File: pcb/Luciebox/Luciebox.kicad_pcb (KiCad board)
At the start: 2 copper layers, 100 x 100 mm, 96 parts, among them J1 Screw_Terminal_01x07, J2 Screw_Terminal_01x07, J3 Screw_Terminal_01x07, J4 Screw_Terminal_01x07, J5 Screw_Terminal_01x07, P1 CONN_01X01, P2 CONN_01X01, P3 CONN_01X01, P4 CONN_01X01, P5 Digital, P6 Power, P7 Digital, P8 Analog, Q1 BC558, Q2 N-Channel_Mosfet, T1 terminal_13x1, T10 terminal_8x1, T11 terminal_3x1, T2 terminal_8x1, T3 terminal_8x1, T4 terminal_8x1, T5 terminal_8x1, T6 terminal_8x1, T7 terminal_8x1, T8 terminal_8x1, T9 terminal_8x1, U1 CA56-12SRWA, U2 ULN2003A, U3 ATmega328-PU, U4 8X8PADS, Y1 16MHz

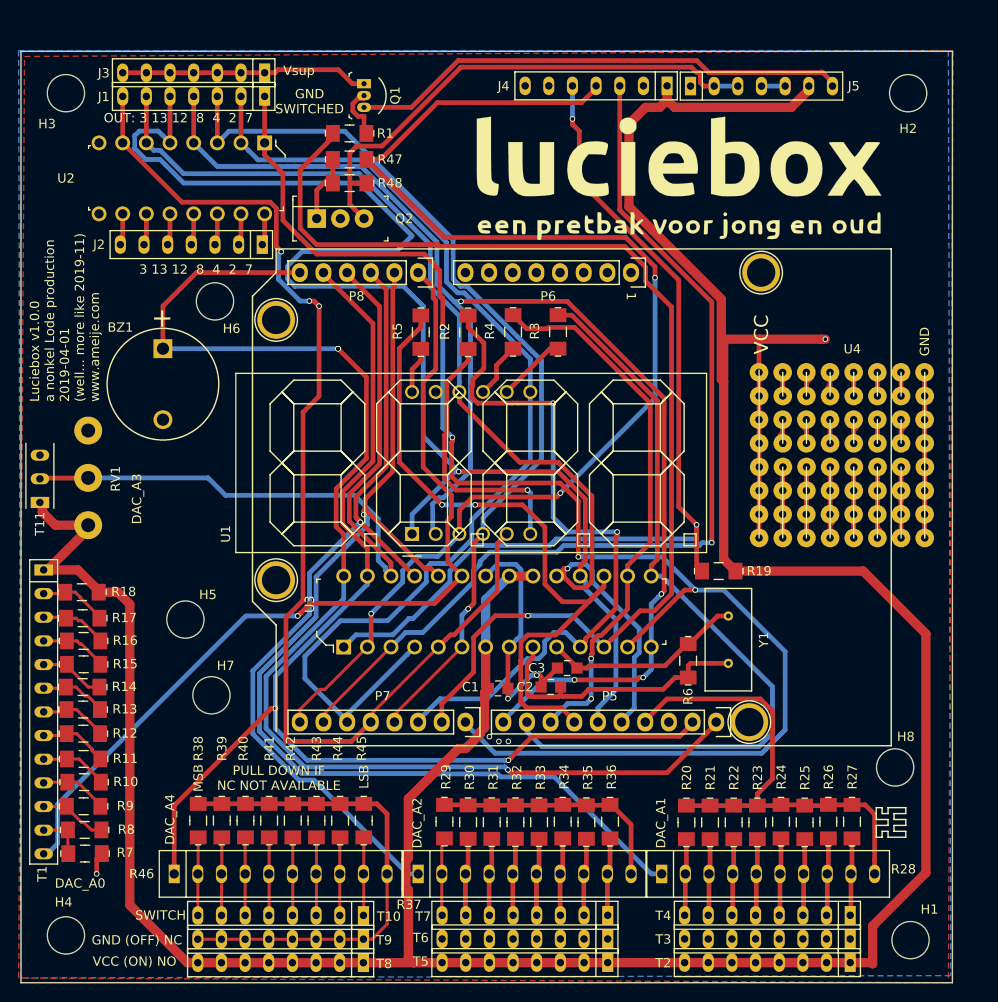
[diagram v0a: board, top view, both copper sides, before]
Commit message: reload autosave, the v1.0.0 save was not actually saved. oioioi. So, now at v1.0.0 pcb!
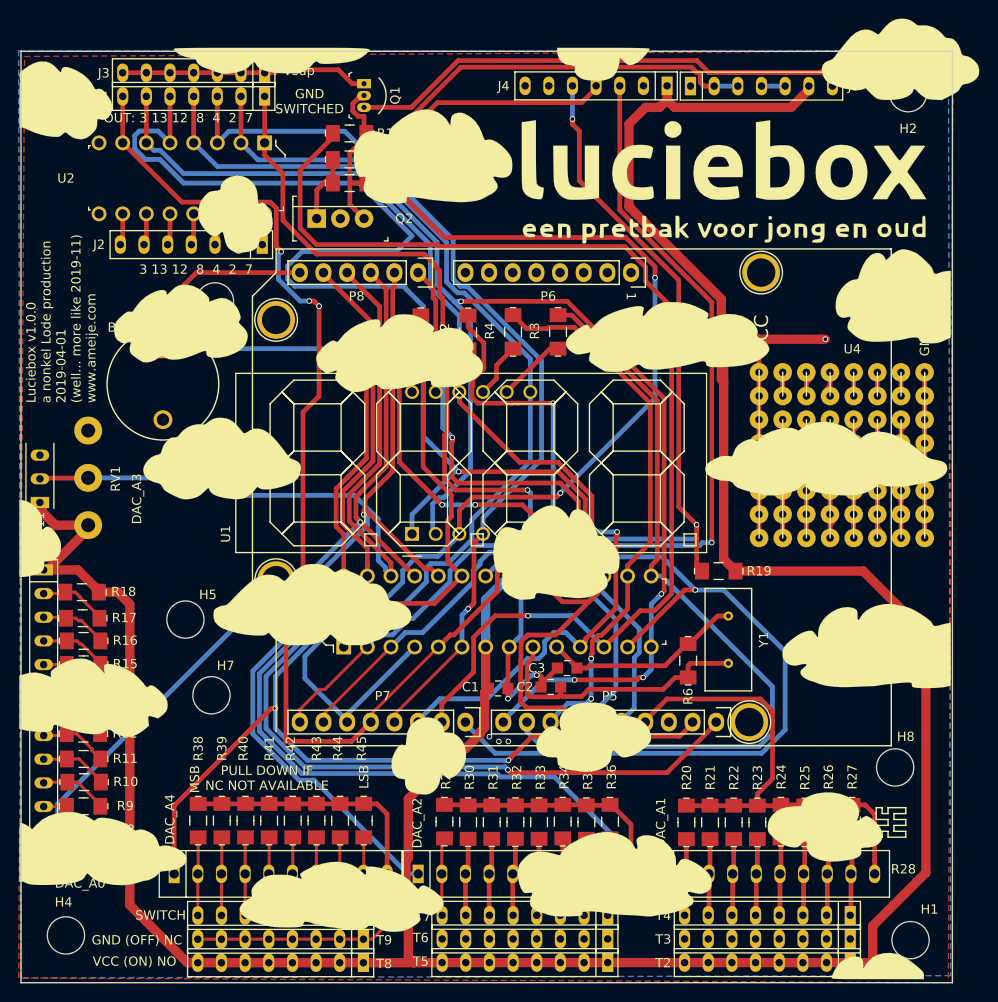
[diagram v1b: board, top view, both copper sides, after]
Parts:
- removed the G*** at (50.3, 49.9)
- added G***: LOGO, artwork:sky_with_clouds_negative_adapted_silk, F.Cu at (50.0, 49.8)
- moved G*** 4.84 mm to (59.4, 45.2)
